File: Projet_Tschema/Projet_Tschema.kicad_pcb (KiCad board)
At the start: 2 copper layers, 41 parts, among them J1 Raspberry_Pi_2_3, J2 Screw_Terminal_01x02, J3 Conn_D42V55F5, U1 SC16IS-752, U2 AMS1117, Y1 14.7456M

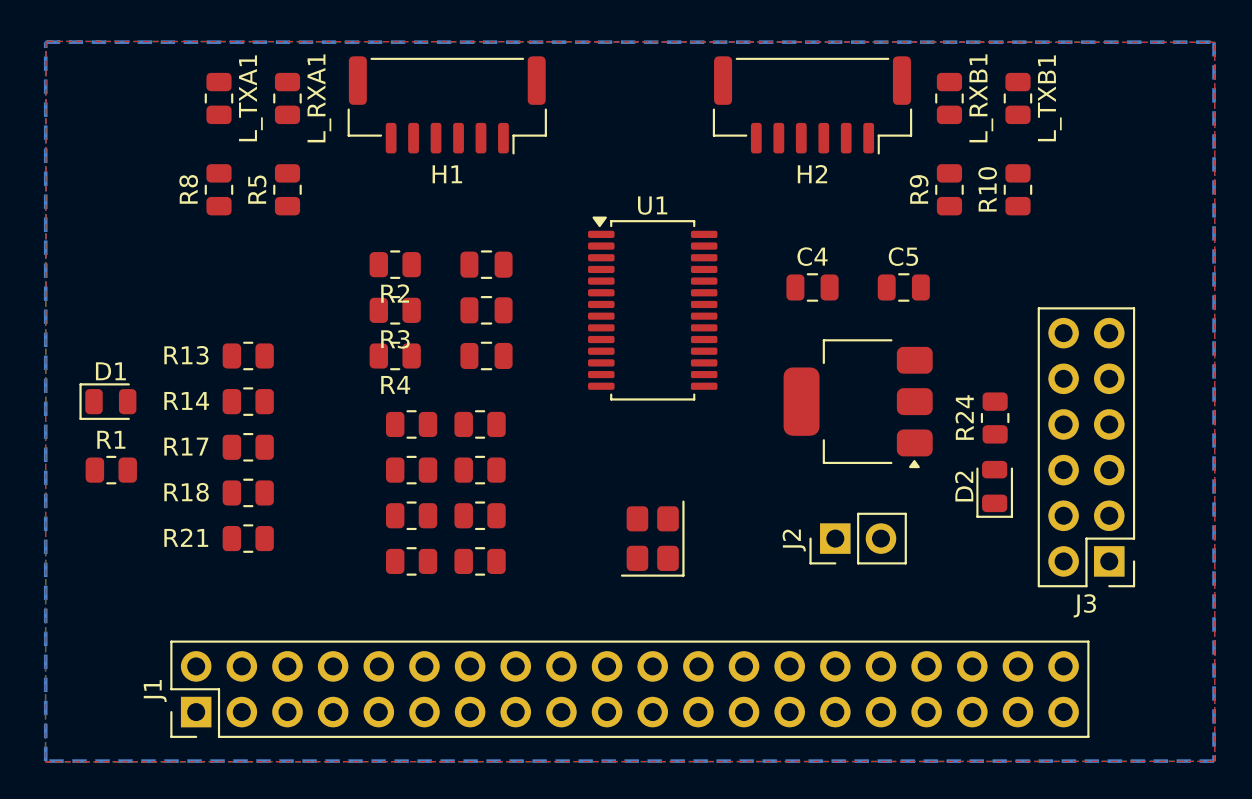
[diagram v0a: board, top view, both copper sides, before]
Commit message: first version finished
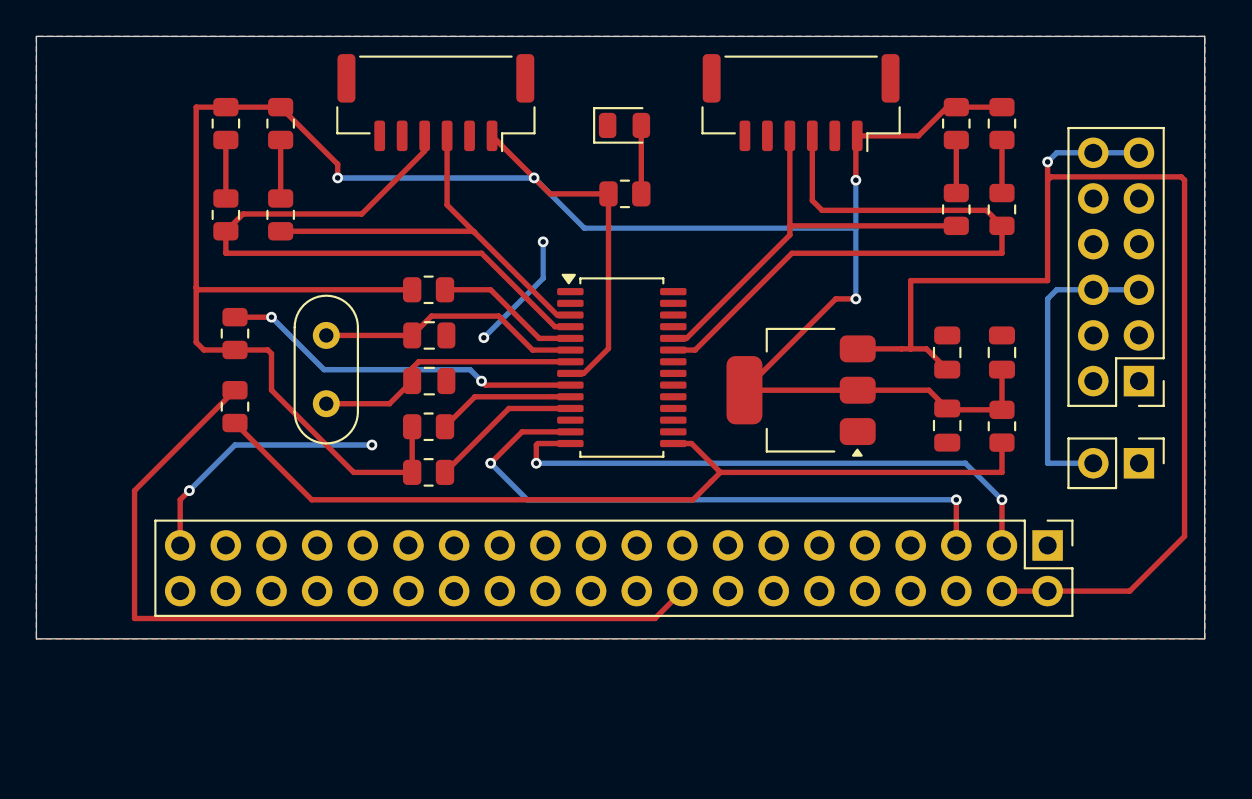
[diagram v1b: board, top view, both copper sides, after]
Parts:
- removed D2: LED_Filled, LED_SMD:LED_0805_2012Metric
- removed R14, R15, R16, R17, R18, R19, R20, R21, R22, R23: NC, Resistor_SMD:R_0805_2012Metric
- removed R24: 1K, Resistor_SMD:R_0805_2012Metric
- Y1: footprint Crystal:Crystal_SMD_3225-4Pin_3.2x2.5mm -> Crystal:Crystal_HC52-U_Vertical
- moved J1 48.3 mm to (175.6, 109.6), turned to -90 degrees
- moved R3 34.4 mm to (173.1, 103.0), turned to -90 degrees
- moved D1 32.4 mm to (152.1, 86.2)
- moved R1 32.4 mm to (152.1, 90.0)
- moved C1 28.7 mm to (173.1, 98.9), turned to -90 degrees
- moved Y1 19.6 mm to (135.5, 101.7)
- moved J2 17.4 mm to (180.7, 105.0), turned to -90 degrees
- moved C4 10.7 mm to (170.1, 102.9), turned to -90 degrees
- moved J3 10.2 mm to (180.7, 100.5)
- moved R4 9.00 mm to (130.4, 97.8), turned to 90 degrees
- moved L_RXA1 7.33 mm to (129.9, 91.2), turned to 90 degrees
- moved L_TXA1 7.33 mm to (133.0, 91.2), turned to 90 degrees
- moved L_TXB1 6.24 mm to (173.1, 90.9), turned to 90 degrees
- moved L_RXB1 6.19 mm to (170.6, 90.9), turned to 90 degrees
- moved C2 5.06 mm to (141.2, 97.9), turned to 0 degrees
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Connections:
- H1 pad 5: /RTSA -> unconnected-(H1-Pin_5-Pad5)
- H1 pad 6: /CTSA -> unconnected-(H1-Pin_6-Pad6)
- H2 pad 5: /RTSB -> unconnected-(H2-Pin_5-Pad5)
- H2 pad 6: /CTSB -> unconnected-(H2-Pin_6-Pad6)
- J1 pad 15: /P22 -> unconnected-(J1-GPIO3-Pad15)
- J1 pad 16: /P23 -> unconnected-(J1-GPIO4-Pad16)
- J1 pad 38: /P20 -> unconnected-(J1-GPIO28-Pad38)
- J1 pad 40: /P21 -> unconnected-(J1-GPIO29-Pad40)
- J3 pad 1: Net-(J3-Pin_1) -> unconnected-(J3-Pin_1-Pad1)
- J3 pad 11: GND -> /5V
- J3 pad 3: /Vin -> unconnected-(J3-Pin_3-Pad3)
- J3 pad 4: GND -> unconnected-(J3-Pin_4-Pad4)
- J3 pad 5: GND -> /Vin
- J3 pad 6: /5V -> /Vin
- J3 pad 7: unconnected-(J3-Pin_7-Pad7) -> GND
- J3 pad 8: unconnected-(J3-Pin_8-Pad8) -> GND
- J3 pad 9: /Vin -> GND
- U1 pad 1: /RTSA -> unconnected-(U1-~{RTSA}-Pad1)
- U1 pad 16: /CTSB -> unconnected-(U1-~{CTSB}-Pad16)
- U1 pad 17: /RTSB -> unconnected-(U1-~{RTSB}-Pad17)
- U1 pad 2: /CTSA -> unconnected-(U1-~{CTSA}-Pad2)
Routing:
- net /3V3: track 0.00 -> 146.3 mm, vias 0 -> 4
- net /5V: track 0.00 -> 67.8 mm, vias 0 -> 1
- net /IRQ: track 0.00 -> 50.0 mm
- net /P24: track 0.00 -> 46.1 mm
- net /TXDB: track 0.00 -> 36.8 mm
- net /RXDA: track 0.00 -> 35.8 mm
- net /P_SCL: track 0.00 -> 34.4 mm, vias 0 -> 2
- net /P_SDA: track 0.00 -> 32.2 mm, vias 0 -> 2
- net /TXDA: track 0.00 -> 24.1 mm
- net /RXDB: track 0.00 -> 23.6 mm
- net GND: track 0.00 -> 21.2 mm, vias 0 -> 4
- net Net-(U1-I2C/~{SPI}): track 0.00 -> 20.2 mm, vias 0 -> 2
- net /Vin: track 0.00 -> 17.0 mm
- net Net-(U1-XTAL2): track 0.00 -> 15.0 mm
- net Net-(U1-XTAL1): track 0.00 -> 14.8 mm
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- added copper zone on B.Cu, net GND
- added copper zone on F.Cu, net GND
- removed copper zone on B.Cu, net (none)
- removed copper zone on F.Cu, net (none)
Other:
- board outline added: 65 x 33.5 mm
